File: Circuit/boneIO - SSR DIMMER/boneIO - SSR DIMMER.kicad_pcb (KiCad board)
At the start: 2 copper layers, 197 x 102 mm, 209 parts, among them J1 Conn_02x04_Odd_Even, J10 Screw_Terminal_01x04, J11 Screw_Terminal_01x04, J12 Screw_Terminal_01x04, J13 Screw_Terminal_01x04, J2 DIMMER, J3 DIMMER, J4 DIMMER, J5 DIMMER, J6 DIMMER, J7 DIMMER, J8 Screw_Terminal_01x04, J9 Screw_Terminal_01x04, Q1 BT136-600, Q10 BT136-600, Q11 BT136-600, Q12 BT136-600, Q13 BTA12-600B, Q14 BTA12-600B, Q15 BTA12-600B, Q16 BTA12-600B, Q17 BTA12-600B, Q18 BTA12-600B, Q19 BTA12-600B, Q2 BT136-600, Q20 BTA12-600B, Q21 BTA12-600B, Q22 BTA12-600B, Q23 BTA12-600B, Q24 BTA12-600B, Q3 BT136-600, Q4 BT136-600, Q5 BT136-600, Q6 BT136-600, Q7 BT136-600, Q8 BT136-600, Q9 BT136-600, U1 MCP9808-E_SO8, U10 MOC3041M, U11 MOC3041M, U12 MOC3041M, U13 MOC3041M, U14 MOC3041M, U15 MOC3041M, U16 MOC3041M, U17 MOC3041M, U18 MOC3041M, U19 MOC3041M, U2 MCP9808-E_MS, U20 MOC3041M, U21 MOC3041M, U22 MOC3041M, U23 MOC3041M, U24 MOC3041M, U25 MOC3041M, U26 MOC3041M, U27 MOC3041M, U28 MOC3041M, U29 MOC3041M, U3 PCA9685PW, U30 MOC3041M, U31 MOC3041M, U4 MOC3041M, U5 ULN2803A, U6 ULN2803A, U7 MOC3041M, U8 MCP23017_SS

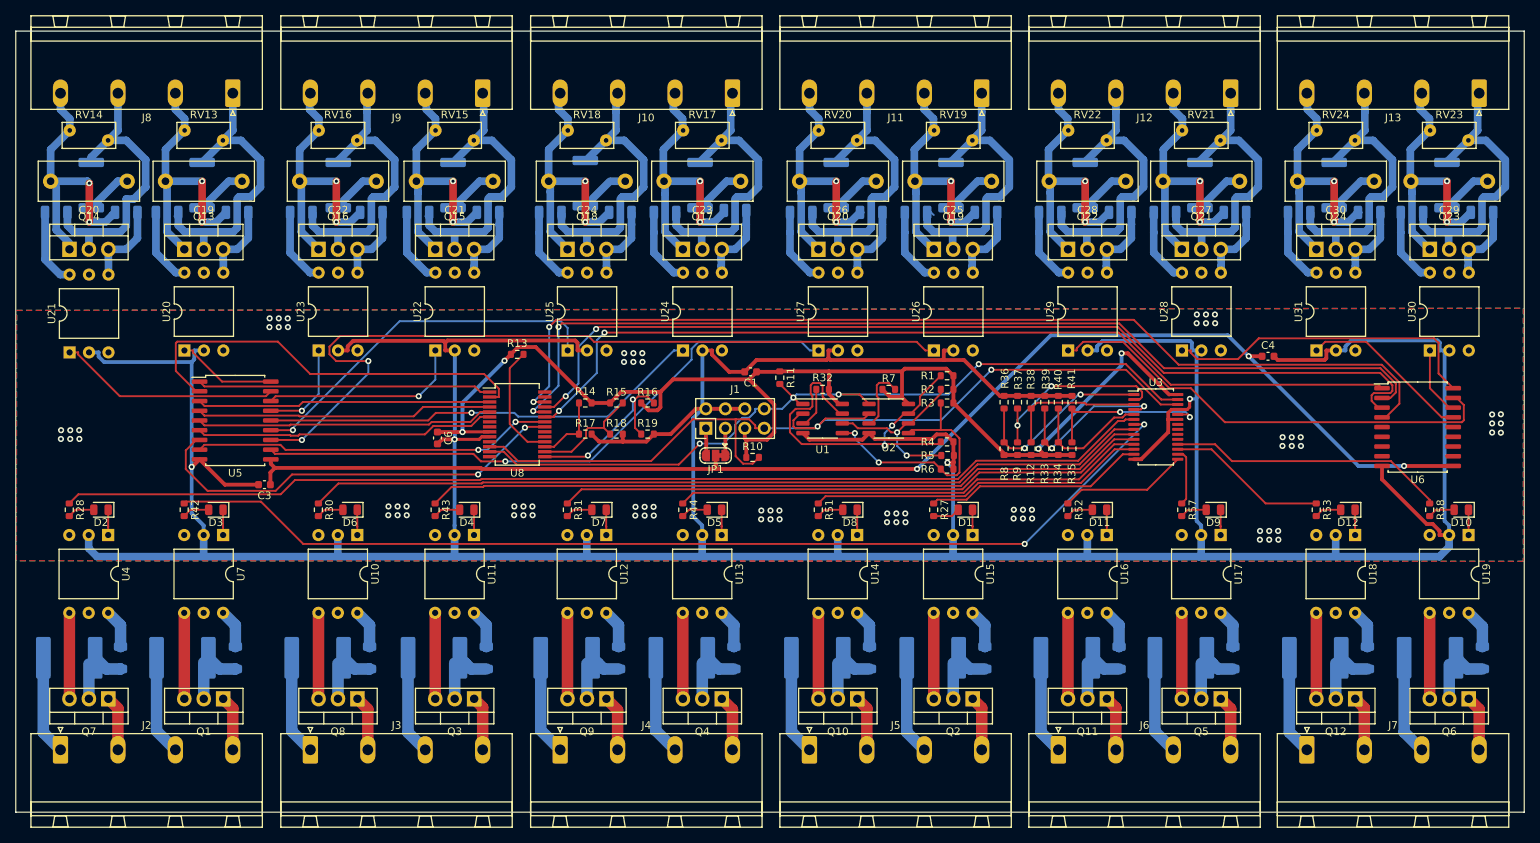
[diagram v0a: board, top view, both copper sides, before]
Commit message: Add files via upload
Poprawione
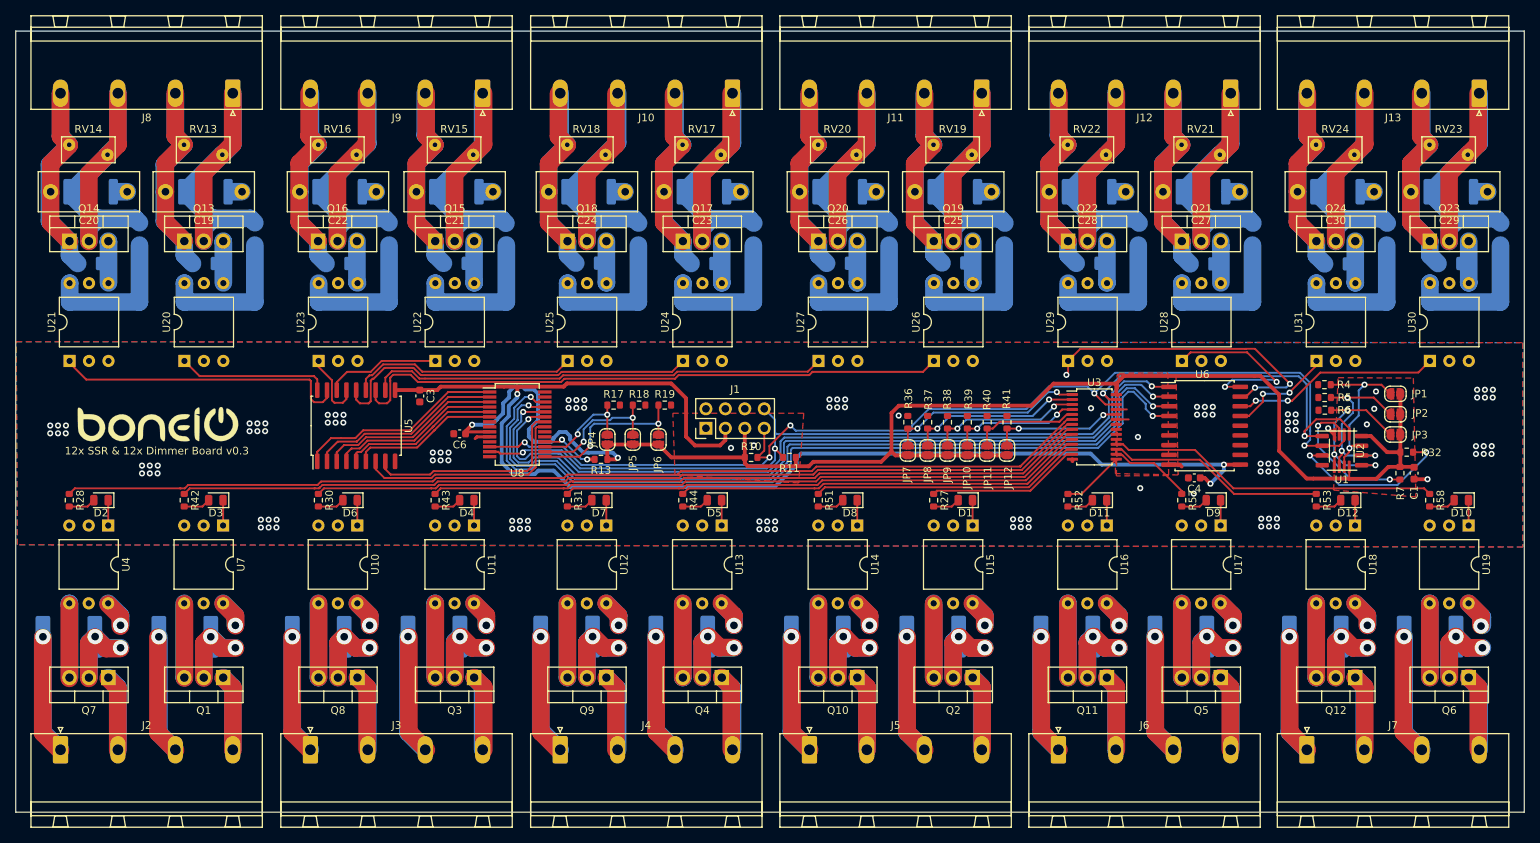
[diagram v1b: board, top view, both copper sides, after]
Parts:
- removed R1, R14, R15, R2, R3: 0k_NC, Resistor_SMD:R_0603_1608Metric
- removed R12, R16, R33, R34, R35, R8, R9: 0k, Resistor_SMD:R_0603_1608Metric
- added G***: LOGO, Symbol:boneIO_LOGO_srednie, F.Cu at (66.9, 88.7)
- added JP10: Jumper_NO_Small, Jumper:SolderJumper-2_P1.3mm_Open_RoundedPad1.0x1.5mm, F.Cu at (172.6, 92.0)
- added JP11: Jumper_NO_Small, Jumper:SolderJumper-2_P1.3mm_Open_RoundedPad1.0x1.5mm, F.Cu at (175.2, 92.0)
- added JP12: Jumper_NO_Small, Jumper:SolderJumper-2_P1.3mm_Open_RoundedPad1.0x1.5mm, F.Cu at (177.7, 92.0)
- added JP2: Jumper_NO_Small, Jumper:SolderJumper-2_P1.3mm_Open_RoundedPad1.0x1.5mm, F.Cu at (228.5, 87.3)
- added JP3: Jumper_NO_Small, Jumper:SolderJumper-2_P1.3mm_Open_RoundedPad1.0x1.5mm, F.Cu at (228.5, 90.0)
- added JP4: Jumper_NO_Small, Jumper:SolderJumper-2_P1.3mm_Open_RoundedPad1.0x1.5mm, F.Cu at (125.6, 90.6)
- added JP5: Jumper_NO_Small, Jumper:SolderJumper-2_P1.3mm_Open_RoundedPad1.0x1.5mm, F.Cu at (128.9, 90.6)
- added JP6: Jumper_NO_Small, Jumper:SolderJumper-2_P1.3mm_Open_RoundedPad1.0x1.5mm, F.Cu at (132.2, 90.6)
- added JP7: Jumper_NO_Small, Jumper:SolderJumper-2_P1.3mm_Open_RoundedPad1.0x1.5mm, F.Cu at (164.8, 92.0)
- added JP8: Jumper_NO_Small, Jumper:SolderJumper-2_P1.3mm_Open_RoundedPad1.0x1.5mm, F.Cu at (167.4, 92.0)
- added JP9: Jumper_NO_Small, Jumper:SolderJumper-2_P1.3mm_Open_RoundedPad1.0x1.5mm, F.Cu at (170.0, 92.0)
- JP1: value SolderJumper_3_Bridged12 -> Jumper_NO_Small; footprint Jumper:SolderJumper-3_P1.3mm_Bridged12_RoundedPad1.0x1.5mm -> Jumper:SolderJumper-2_P1.3mm_Open_RoundedPad1.0x1.5mm
- R17, R18, R36, R37, R38, R39, R4, R40, R41, R5, R6: value 0k -> 10k
- R19: value 0k_NC -> 10k
- U2: footprint Package_SO:SO-8_3.9x4.9mm_P1.27mm -> Package_SO:MSOP-8_3x3mm_P0.65mm
- moved JP1 89.1 mm to (228.5, 84.7)
- moved C1 87.6 mm to (230.9, 95.0), turned to 270 degrees
- moved R32 76.7 mm to (229.9, 92.3), turned to 0 degrees
- moved U1 67.9 mm to (221.5, 92.1)
- moved R7 67.6 mm to (229.1, 95.0), turned to 270 degrees
- moved U2 59.3 mm to (221.5, 92.1), turned to 270 degrees
- moved R6 49.9 mm to (219.3, 86.8), turned to 180 degrees
- moved R4 49.8 mm to (219.2, 83.5), turned to 180 degrees
- moved R5 49.8 mm to (219.2, 85.1), turned to 180 degrees
- moved U6 27.8 mm to (203.6, 88.8)
- moved C3 23.4 mm to (101.1, 84.9), turned to 270 degrees
- moved C4 18.6 mm to (202.2, 95.6), turned to 180 degrees
- moved R13 17.5 mm to (124.7, 93.2), turned to 180 degrees
- moved U5 15.8 mm to (92.8, 88.8), turned to 90 degrees
- moved R36 12.8 mm to (164.8, 88.4)
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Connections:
- C3 pad 1: VCC -> +5V
- C4 pad 1: VCC -> +5V
- JP1 pad 1: +5V -> +3V3
- JP1 pad 2: VCC -> Net-(JP1-Pad2)
- R4 pad 1: Net-(R1-Pad2) -> Net-(JP1-Pad2)
- U1 pad 7: Net-(R1-Pad2) -> Net-(JP1-Pad2)
- U2 pad 7: Net-(R1-Pad2) -> Net-(JP1-Pad2)
- U5 pad 10: VCC -> +5V
- U6 pad 10: VCC -> +5V
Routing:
- net GND: track 592.0 -> 9.91 mm, vias 82 -> 114
- net VCC: track 175.5 -> 0.00 mm, vias 3 -> 0
- net +5V: track 3.57 -> 168.4 mm, vias 0 -> 3
- net Net-(R1-Pad2): track 48.6 -> 0.00 mm, vias 2 -> 0
- net +3V3: track 166.8 -> 205.0 mm, vias 4 -> 2
- net SDA: track 107.2 -> 143.5 mm
- net K2: track 54.9 -> 25.4 mm
- net K7: track 56.3 -> 29.4 mm, vias 2 -> 0
- net RELAY7: track 104.7 -> 79.2 mm, vias 2 -> 0
- net K10: track 130.0 -> 105.3 mm
- net K12: track 132.7 -> 110.0 mm
- net Net-(JP1-Pad2): track 0.00 -> 21.8 mm, vias 0 -> 2
- net SCL: track 120.4 -> 140.6 mm, vias 2 -> 5
- net RELAY8: track 79.9 -> 59.9 mm, vias 1 -> 0
- net RELAY10: track 60.5 -> 40.6 mm, vias 0 -> 3
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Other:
- board text added: "12x SSR & 12x Dimmer Board v0.3"
